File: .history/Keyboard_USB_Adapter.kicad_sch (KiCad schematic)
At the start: 9 parts, among them J1 USB_C_Receptacle_USB2.0_16P, J2 Conn_01x05, SW1 SW_SPDT, U1 USBLC6-2SC6

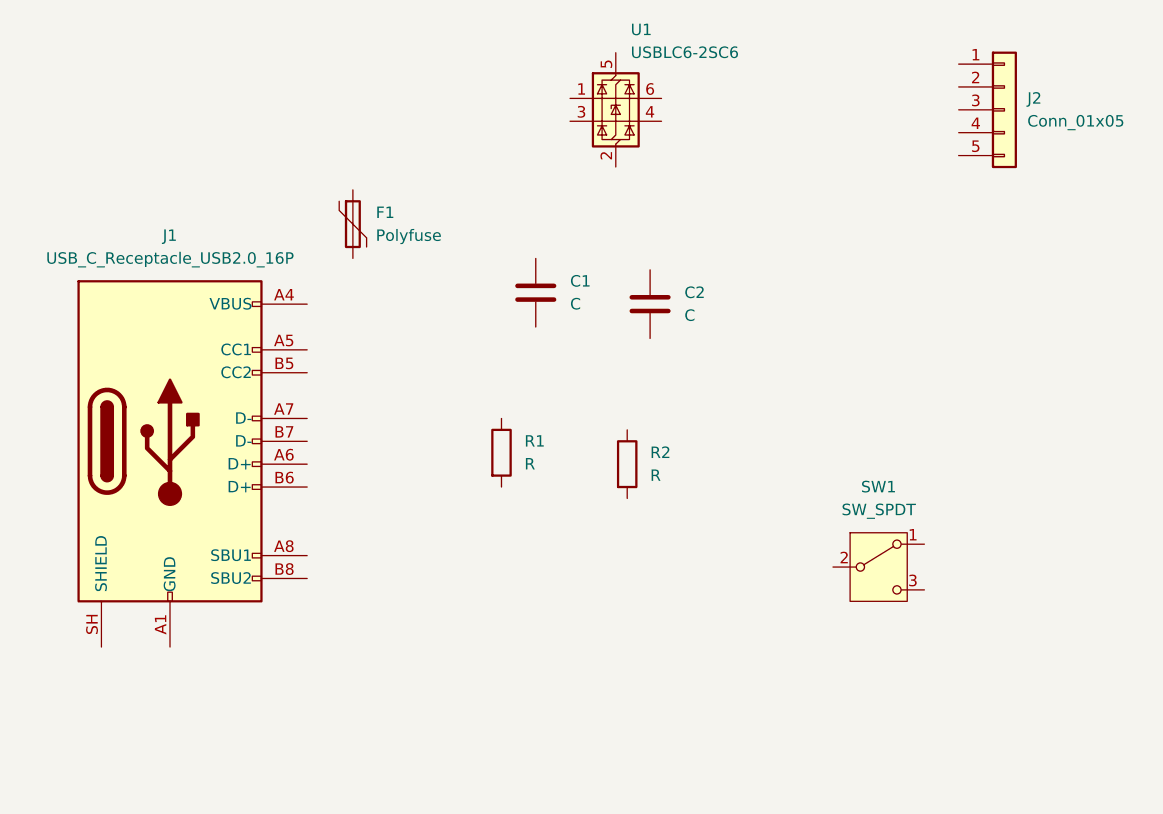
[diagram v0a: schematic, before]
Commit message: placed parts
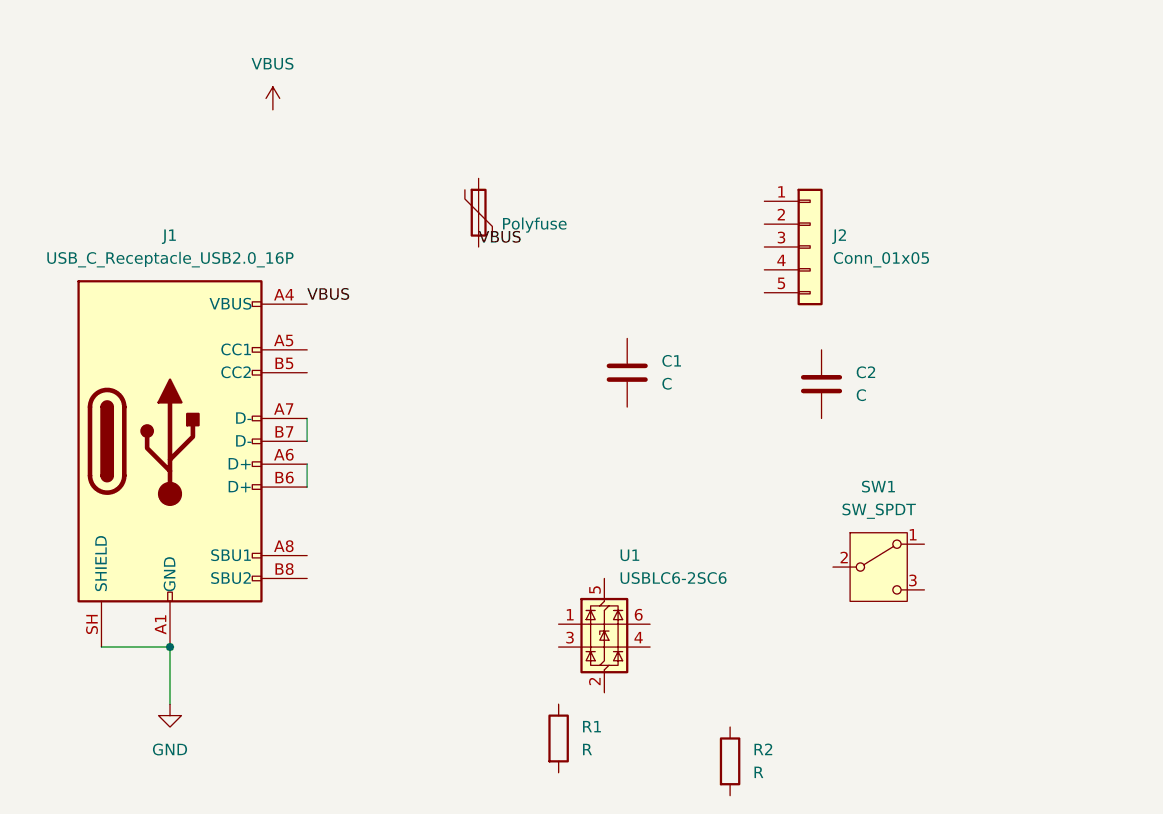
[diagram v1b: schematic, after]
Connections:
- net GND: now reaches J1.A1 (GND), J1.A12 (GND), J1.B1 (GND), J1.B12 (GND)
- net GND: now also J1.SH (SHIELD)
- net VBUS: now reaches J1.A4 (VBUS), J1.A9 (VBUS), J1.B4 (VBUS), J1.B9 (VBUS)
- net VBUS: now also F1.2
- net at J1.A6 (D+): now also J1.B6 (D+)
- net at J1.A7 (D-): now also J1.B7 (D-)
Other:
- moved on the sheet: C1, C2, J2, R1, R2, U1

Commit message: Progress
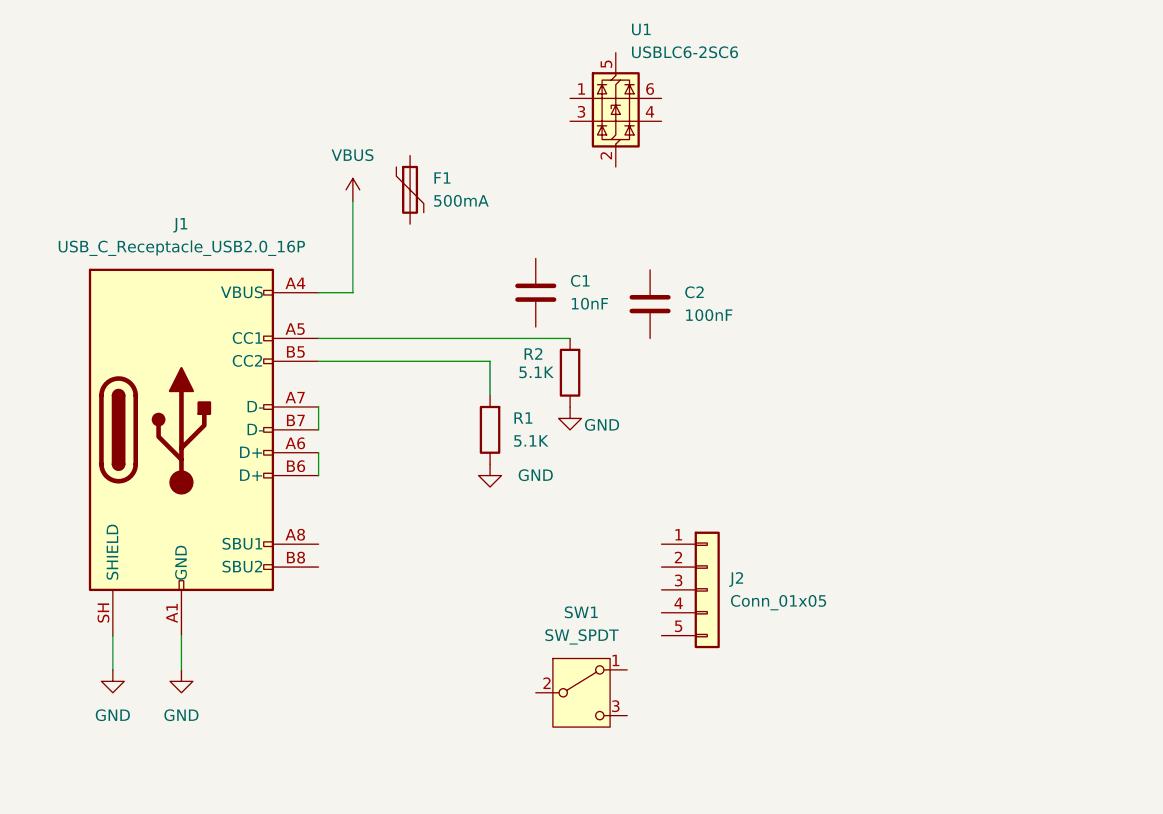
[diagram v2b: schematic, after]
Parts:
- C1: value C -> 10nF
- C2: value C -> 100nF
- F1: value Polyfuse -> 500mA
- R1, R2: value R -> 5.1K
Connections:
- net GND: now also R1.1, R2.1
- net VBUS: no longer F1.2
- net at J1.A5 (CC1): now also R2.2
- net at J1.B5 (CC2): now also R1.2
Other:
- moved on the sheet: C1, C2, J1, J2, R1, R2, SW1, U1
